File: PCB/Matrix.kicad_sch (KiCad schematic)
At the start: 192 parts, among them J1 USB_C_Receptacle_USB2.0_14P, J2 Conn_01x03_Pin, J3 Conn_01x13_Pin, J4 Conn_01x06_Pin, J5 Conn_01x04_Pin, J6 Conn_01x03_Pin, SW1 Switch, U1 RP2040, U2 NCP1117-3.3_SOT223, U3 W25Q128JVS, U4 IS31FL3737, Y1 Crystal_GND24

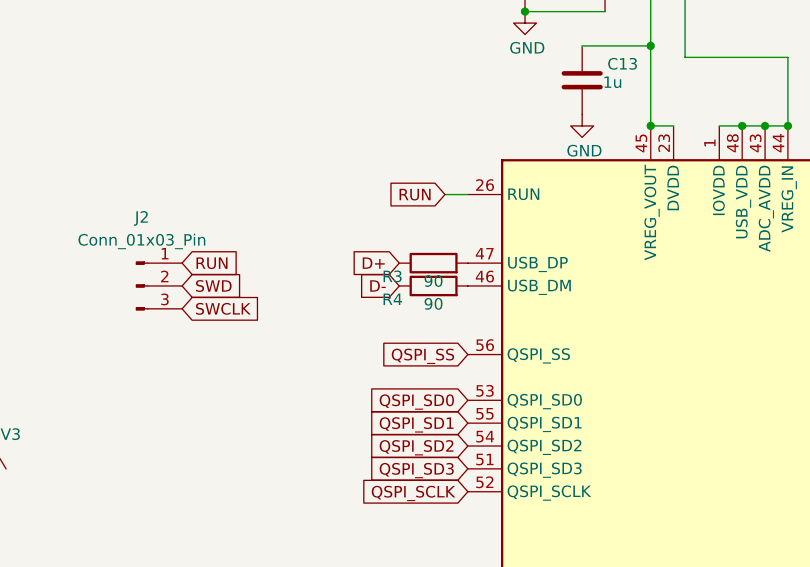
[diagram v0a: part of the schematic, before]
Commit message: Add files via upload
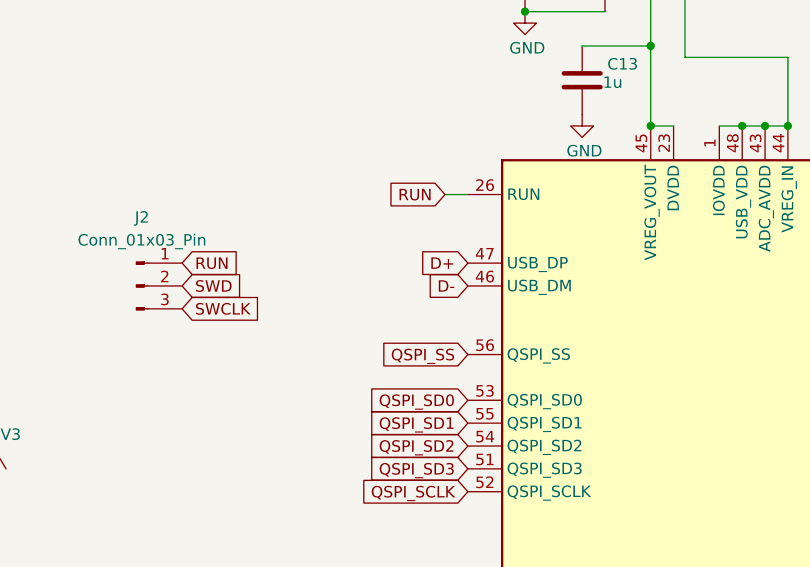
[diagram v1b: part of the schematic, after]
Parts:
- removed R3, R4: 90, Resistor_SMD:R_0402_1005Metric, symbol Device:R
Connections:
- net D+: now also U1.47 (USB_DP)
- net D-: now also U1.46 (USB_DM)
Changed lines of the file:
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@@
 	(global_label "D-"
 		(shape input)
-		(at 269.24 55.88 180)
+		(at 276.86 55.88 180)
 		(fields_autoplaced yes)
 		(effects
@@
 		)
 		(property "Intersheetrefs" "${INTERSHEET_REFS}"
-			(at 263.4124 55.88 0)
+			(at 271.0324 55.88 0)
 			(effects
 				(font
@@
 	(global_label "D+"
 		(shape input)
-		(at 269.24 53.34 180)
+		(at 276.86 53.34 180)
 		(fields_autoplaced yes)
 		(effects
@@
 		)
 		(property "Intersheetrefs" "${INTERSHEET_REFS}"
-			(at 263.4124 53.34 0)
+			(at 271.0324 53.34 0)
 			(effects
 				(font
@@
 	(symbol
 		(lib_id "Device:R")
-		(at 273.05 55.88 90)
-		(unit 1)
-		(exclude_from_sim no)
-		(in_bom yes)
-		(on_board yes)
-		(dnp no)
-		(property "Reference" "R4"
-			(at 268.478 57.404 90)
-			(effects
-				(font
-					(size 1.27 1.27)
-				)
-			)
-		)
-		(property "Value" "90"
-			(at 273.05 57.912 90)
-			(effects
-				(font
-					(size 1.27 1.27)
-				)
-			)
-		)
-		(property "Footprint" "Resistor_SMD:R_0402_1005Metric"
-			(at 273.05 57.658 90)
-			(effects
-				(font
-					(size 1.27 1.27)
-				)
-				(hide yes)
-			)
-		)
-		(property "Datasheet" "~"
-			(at 273.05 55.88 0)
-			(effects
-				(font
-					(size 1.27 1.27)
-				)
-				(hide yes)
-			)
-		)
-		(property "Description" "Resistor"
-			(at 273.05 55.88 0)
-			(effects
-				(font
-					(size 1.27 1.27)
-				)
-				(hide yes)
-			)
-		)
-		(pin "2"
-		)
-		(pin "1"
-		)
-		(instances
-			(project "Matrix"
-				(path "/36e18e2e-f10f-498a-b319-82b0e6fc74a4"
-					(reference "R4")
-					(unit 1)
-				)
-			)
-		)
-	)
-	(symbol
-		(lib_id "Device:R")
 		(at 287.02 176.53 180)
 		(unit 1)
@@
 					(unit 1)
 				)
-			)
-		)
-	)
-	(symbol
-		(lib_id "Device:R")
-		(at 273.05 53.34 90)
-		(unit 1)
-		(exclude_from_sim no)
-		(in_bom yes)
-		(on_board yes)
-		(dnp no)
-		(property "Reference" "R3"
-			(at 268.478 54.864 90)
-			(effects
-				(font
-					(size 1.27 1.27)
-				)
-			)
-		)
-		(property "Value" "90"
-			(at 273.05 55.372 90)
-			(effects
-				(font
-					(size 1.27 1.27)
-				)
-			)
-		)
-		(property "Footprint" "Resistor_SMD:R_0402_1005Metric"
-			(at 273.05 55.118 90)
-			(effects
-				(font
-					(size 1.27 1.27)
-				)
-				(hide yes)
-			)
-		)
-		(property "Datasheet" "~"
-			(at 273.05 53.34 0)
-			(effects
-				(font
-					(size 1.27 1.27)
-				)
-				(hide yes)
-			)
-		)
-		(property "Description" "Resistor"
-			(at 273.05 53.34 0)
-			(effects
-				(font
-					(size 1.27 1.27)
-				)
-				(hide yes)
-			)
-		)
-		(pin "2"
-		)
-		(pin "1"
-		)
-		(instances
-			(project "Matrix"
-				(path "/36e18e2e-f10f-498a-b319-82b0e6fc74a4"
-					(reference "R3")
-					(unit 1)
-				)
